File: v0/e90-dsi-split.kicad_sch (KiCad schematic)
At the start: 15 parts, among them J1 3-2328724-1, J2 BM23PF0.8-40DP-0.35V_51_, J3 I2C Pinstack, J4 GPIO Pinstack

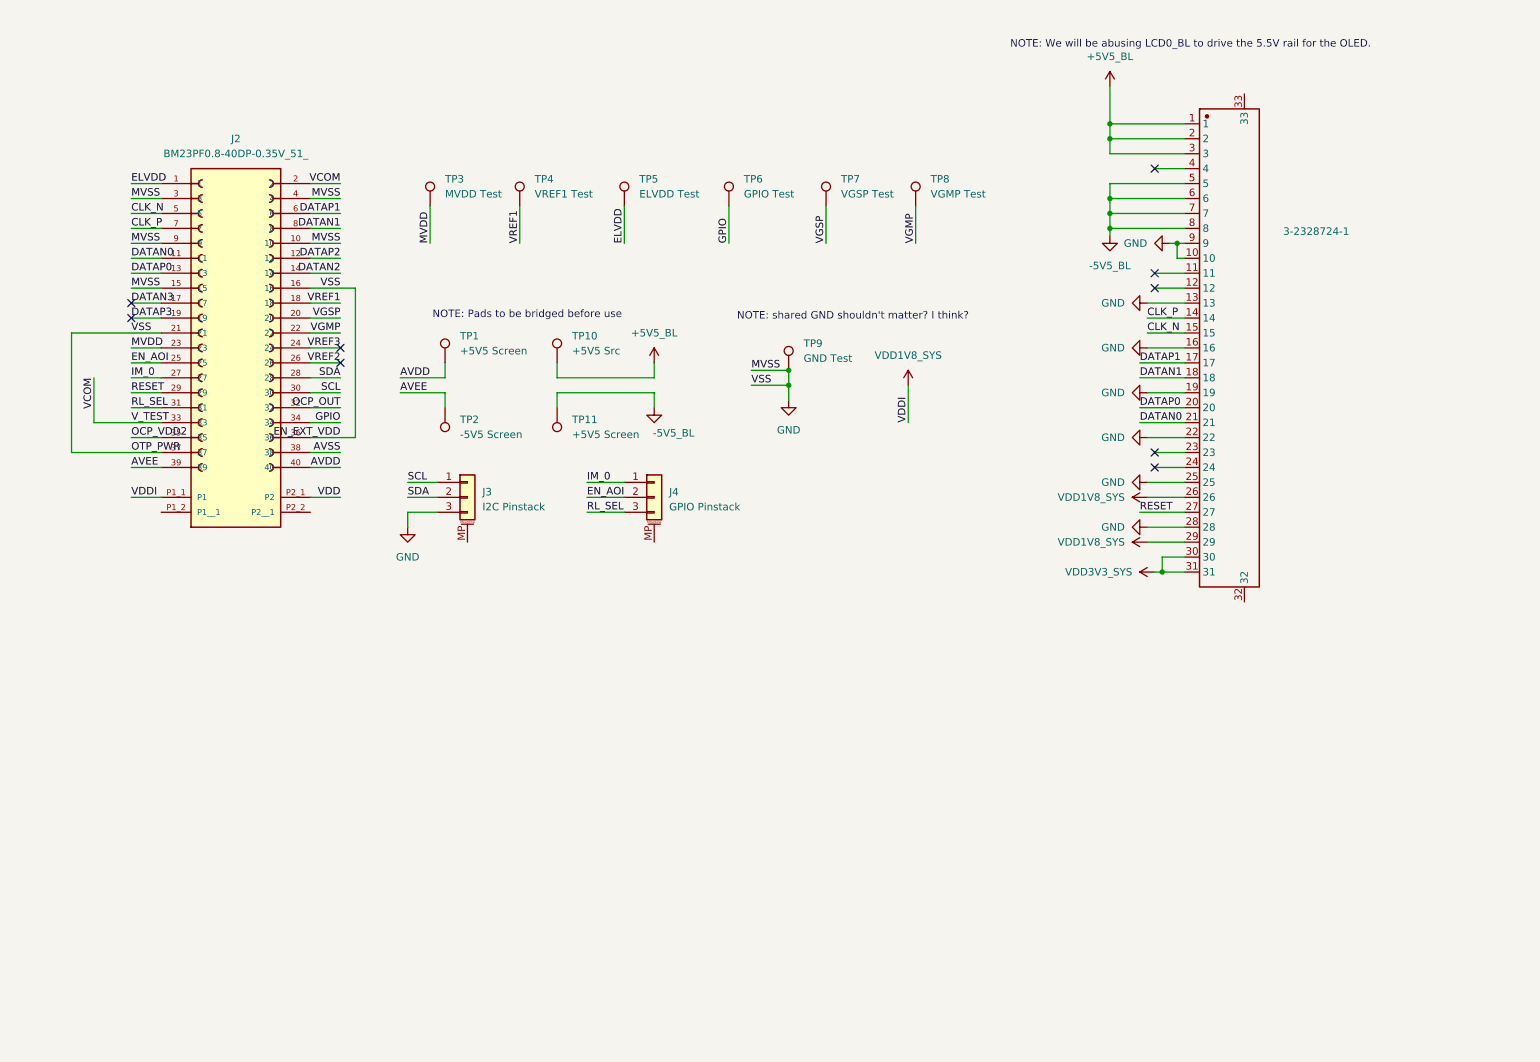
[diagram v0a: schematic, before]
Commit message: v1
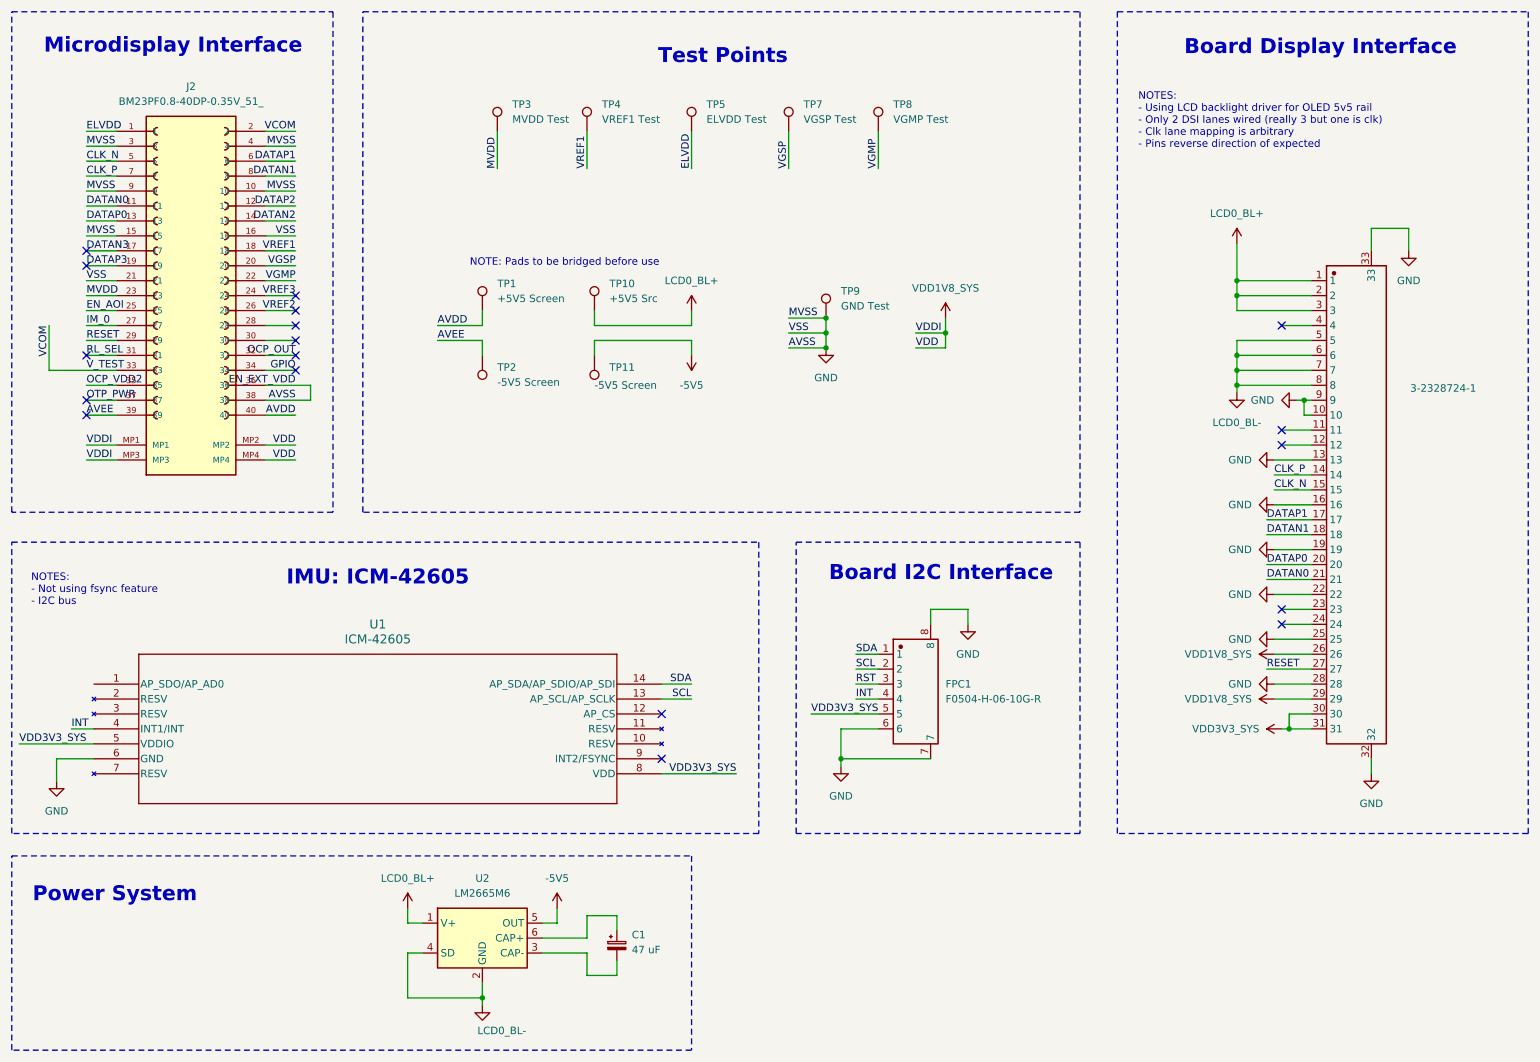
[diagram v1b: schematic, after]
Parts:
- removed J3: I2C Pinstack, Connector_PinHeader_1.00mm:PinHeader_1x03_P1.00mm_Horizontal, symbol Connector_Generic_MountingPin:Conn_01x03_MountingPin
- removed J4: GPIO Pinstack, Connector_PinHeader_1.00mm:PinHeader_1x03_P1.00mm_Horizontal, symbol Connector_Generic_MountingPin:Conn_01x03_MountingPin
- removed TP6: GPIO Test, TestPoint:TestPoint_Pad_1.0x1.0mm, symbol Connector:TestPoint
- added C1: 47 uF, Capacitor_SMD:C_1206_3216Metric, symbol Device:C_Polarized_Small
- added FPC1: F0504-H-06-10G-R, bacon:FFC-SMD_6P-P0.50_F0504-H-06-10G-R, symbol bacon:F0504-H-06-10G-R
- added U1: ICM-42605, footprints:LGA14_2P5X3X0P91_IVS, symbol 2025-04-06_22-45-15:ICM-42605
- added U2: LM2665M6, Package_TO_SOT_SMD:SOT-23-6, symbol Regulator_SwitchedCapacitor:LM2665M6
- J2: footprint bacon:HRS_BM23PF0.8-40DS-0.35V_51_ -> bacon:BM23PF0840DS035V51-GOOD
- TP11: value +5V5 Screen -> -5V5 Screen
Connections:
- net AVSS is gone; now on net GND: J2.38
- net GND: now also J1.32, J1.33, FPC1.6, FPC1.7, FPC1.8, U1.6 (GND); no longer J2.37
- net SCL: now also FPC1.2, U1.13 (AP_SCL/AP_SCLK); no longer J2.30
- net SDA: now also FPC1.1, U1.14 (AP_SDA/AP_SDIO/AP_SDI); no longer J2.28
- net VDD1V8_SYS: now also J2.MP1, J2.MP2, J2.MP3, J2.MP4; no longer J2.P1_1 (P1)
- net VDD3V3_SYS: now also FPC1.5, U1.5 (VDDIO), U1.8 (VDD)
- net +5V5_BL renamed LCD0_BL+
- net LCD0_BL+: now also U2.1 (V+)
- net -5V5_BL renamed LCD0_BL-
- net LCD0_BL-: now also U2.2 (GND), U2.4 (SD); no longer TP11.1
- removed net VDD: J2.P2_1 (P2)
- new net: C1.2, U2.3 (CAP-)
- new net: C1.1, U2.6 (CAP+)
- new net -5V5: TP11.1, U2.5 (OUT)
- new net INT: FPC1.4, U1.4 (INT1/INT)
- new net OTP_PWR: J2.37
- new net RST: FPC1.3
- no-connect marks 9 -> 18
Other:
- note added: "Board Display Interface"
- note added: "Board I2C Interface"
- note added: "IMU: ICM-42605"
- note added: "Microdisplay Interface"
- note added: "NOTES: - Not using fsync feature - I2C bus"
- note added: "NOTES: - Using LCD backlight driver for OLED 5v5 rail - Only 2 DSI lanes wired (really 3 but one is clk) - Clk lane mapping is arbitrary - Pins reverse direction of expected"
- note added: "Power System"
- note added: "Test Points"
- note removed: "NOTE: We will be abusing LCD0_BL to drive the 5.5V rail for the OLED."
- note removed: "NOTE: shared GND shouldn't matter? I think?"
- moved on the sheet: J2, TP1, TP10, TP11, TP2, TP3, TP4, TP5, TP7, TP8, TP9

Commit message: v1 updates
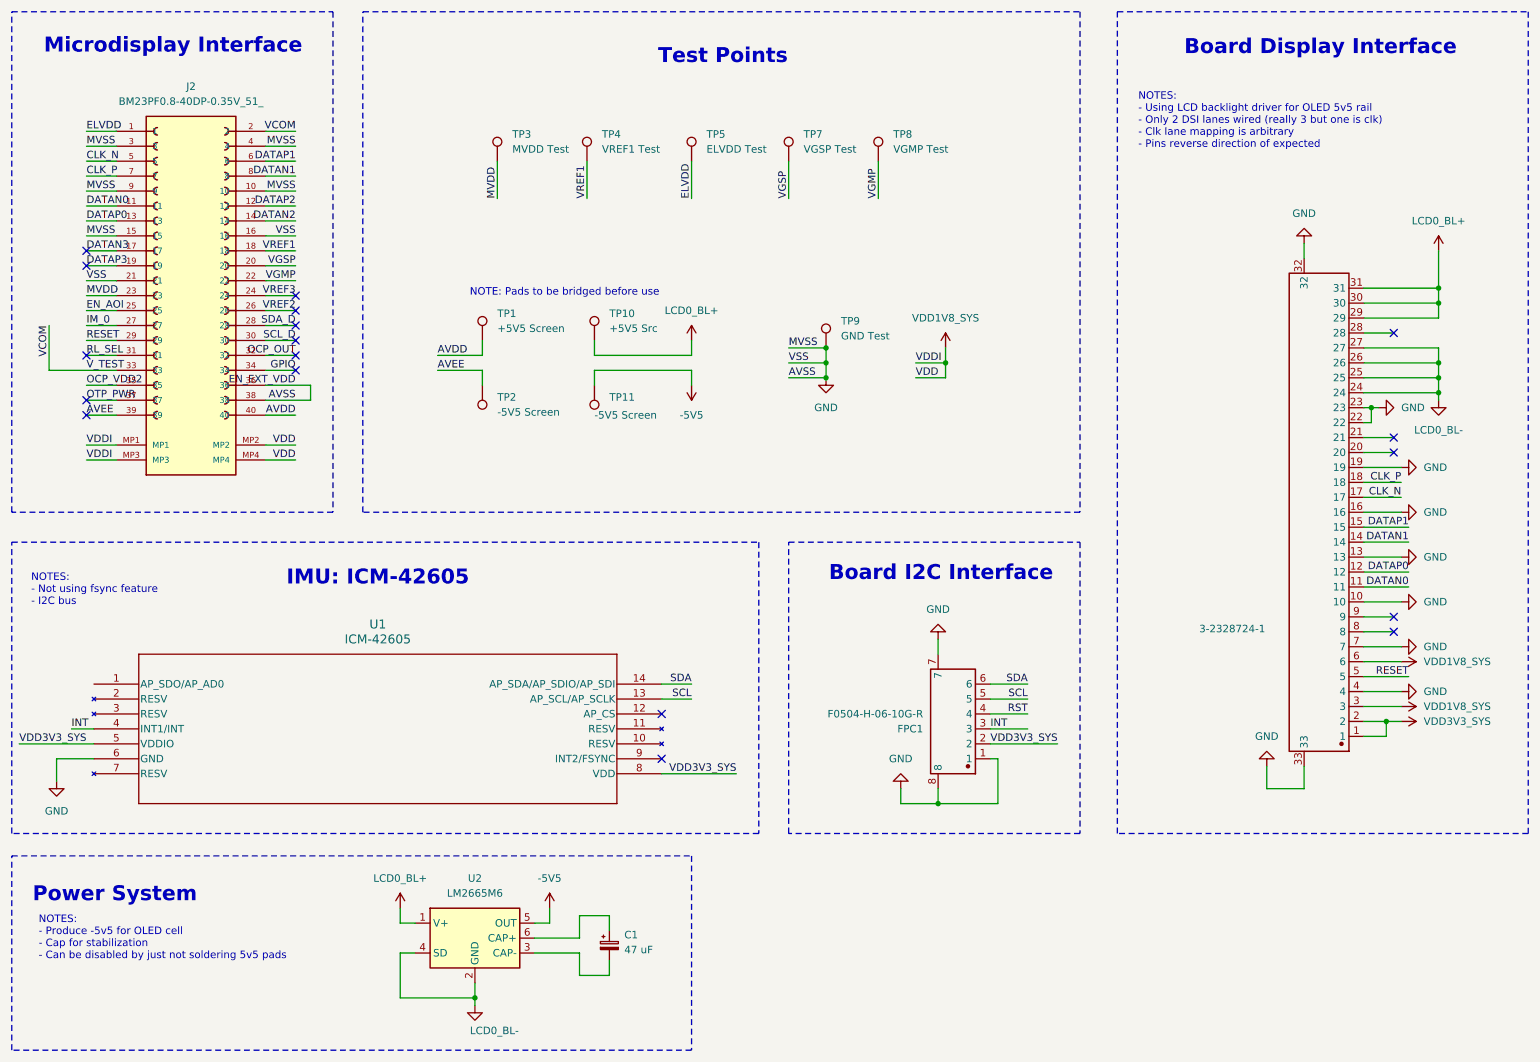
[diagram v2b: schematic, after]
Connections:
- net CLK_N: now also J1.17; no longer J1.15
- net CLK_P: now also J1.18; no longer J1.14
- net DATAN0: now also J1.11; no longer J1.21
- net DATAN1: now also J1.14; no longer J1.18
- net DATAP0: now also J1.12; no longer J1.20
- net DATAP1: now also J1.15; no longer J1.17
- net GND: now also FPC1.1, J1.23, J1.4, J1.7; no longer FPC1.6, J1.25, J1.28, J1.9
- net INT: now also FPC1.3; no longer FPC1.4
- net LCD0_BL+: now also J1.29, J1.30, J1.31; no longer J1.1, J1.2, J1.3
- net LCD0_BL-: now also J1.24, J1.25, J1.26, J1.27; no longer J1.5, J1.6, J1.7, J1.8
- net RESET: now also J1.5; no longer J1.27
- net RST: now also FPC1.4; no longer FPC1.3
- net SCL: now also FPC1.5; no longer FPC1.2
- net SDA: now also FPC1.6; no longer FPC1.1
- net VDD1V8_SYS: now also J1.3, J1.6; no longer J1.26, J1.29
- net VDD3V3_SYS: now also FPC1.2, J1.1, J1.2; no longer FPC1.5, J1.30, J1.31
- net SDA_D: now reaches J2.28
- net SCL_D: now reaches J2.30
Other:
- note added: "NOTES: - Produce -5v5 for OLED cell - Cap for stabilization - Can be disabled by just not soldering 5v5 pads"
- moved on the sheet: C1, FPC1, TP1, TP10, TP11, TP2, TP3, TP4, TP5, TP7, TP8, TP9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

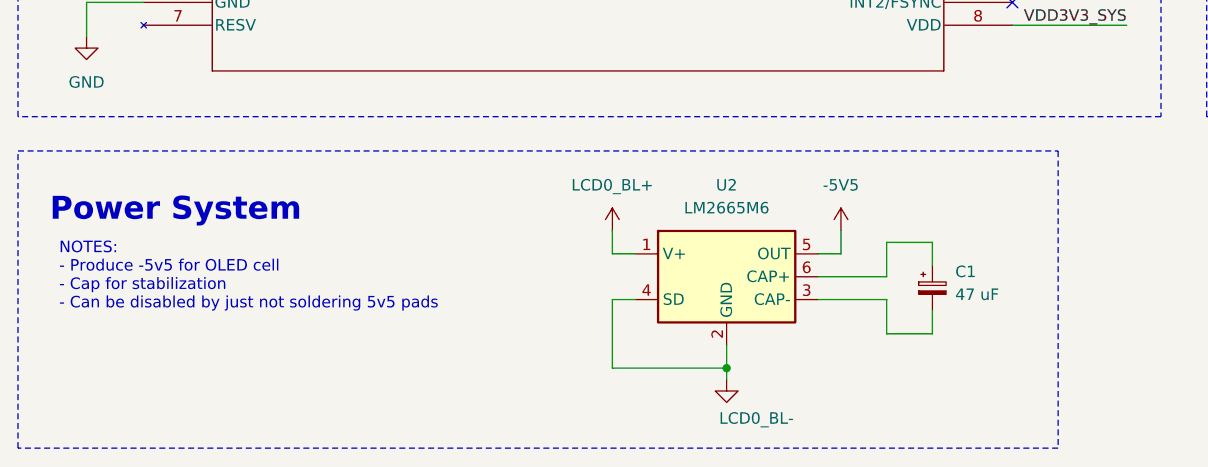
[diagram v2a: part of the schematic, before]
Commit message: v1 updates
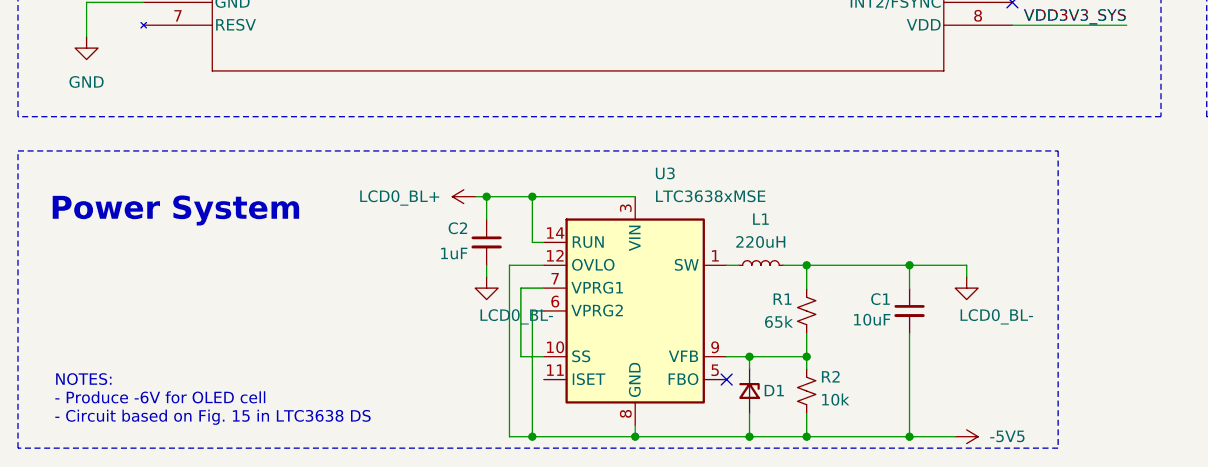
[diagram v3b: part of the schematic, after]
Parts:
- removed C1: 47 uF, Capacitor_SMD:C_1206_3216Metric, symbol Device:C_Polarized_Small
- removed U2: LM2665M6, Package_TO_SOT_SMD:SOT-23-6, symbol Regulator_SwitchedCapacitor:LM2665M6
- added C1: 10uF, Capacitor_SMD:C_1210_3225Metric, symbol Device:C_Small
- added C2: 1uF, Capacitor_SMD:C_0603_1608Metric, symbol Device:C_Small
- added D1: ~, Diode_SMD:D_SOD-123, symbol Device:D_Zener_Small
- added L1: 220uH, Inductor_SMD:L_TDK_NLV32_3.2x2.5mm, symbol Device:L_Small
- added R1: 65k, Resistor_SMD:R_0603_1608Metric, symbol Device:R_Small_US
- added R2: 10k, Resistor_SMD:R_0603_1608Metric, symbol Device:R_Small_US
- added U3: LTC3638xMSE, Package_SO:Analog_MSOP-12-16-1EP_3x4.039mm_P0.5mm_EP1.651x2.845mm, symbol Regulator_Switching:LTC3638xMSE
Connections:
- net -5V5: now also C1.2, D1.2 (A), R2.2, U3.12 (OVLO), U3.16 (GND), U3.17 (GND), U3.6 (VPRG2), U3.8 (GND)
- net LCD0_BL+: now also C2.1, U3.14 (RUN), U3.3 (VIN)
- net LCD0_BL-: now also C1.1, C2.2, L1.2, R1.1
- new net: D1.1 (K), R1.2, R2.1, U3.9 (VFB)
- new net: L1.1, U3.1 (SW)
- new net: U3.10 (SS), U3.7 (VPRG1)
- no-connect marks 18 -> 19
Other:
- note added: "NOTES: - Produce -6V for OLED cell - Circuit based on Fig. 15 in LTC3638 DS"
- note removed: "NOTES: - Produce -5v5 for OLED cell - Cap for stabilization - Can be disabled by just not soldering 5v5 pads"
